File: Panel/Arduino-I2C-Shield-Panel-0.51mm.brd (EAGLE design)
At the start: 127.8 x 141 mm, 136 parts, among them Q1 200mA/50V, Q2 200mA/50V, Q3 200mA/50V, Q4 200mA/50V, Q5 200mA/50V, Q6 200mA/50V, Q7 200mA/50V, Q8 200mA/50V, U1 ARDUINO UNO, U2 ARDUINO UNO, U3 ARDUINO UNO, U4 ARDUINO UNO

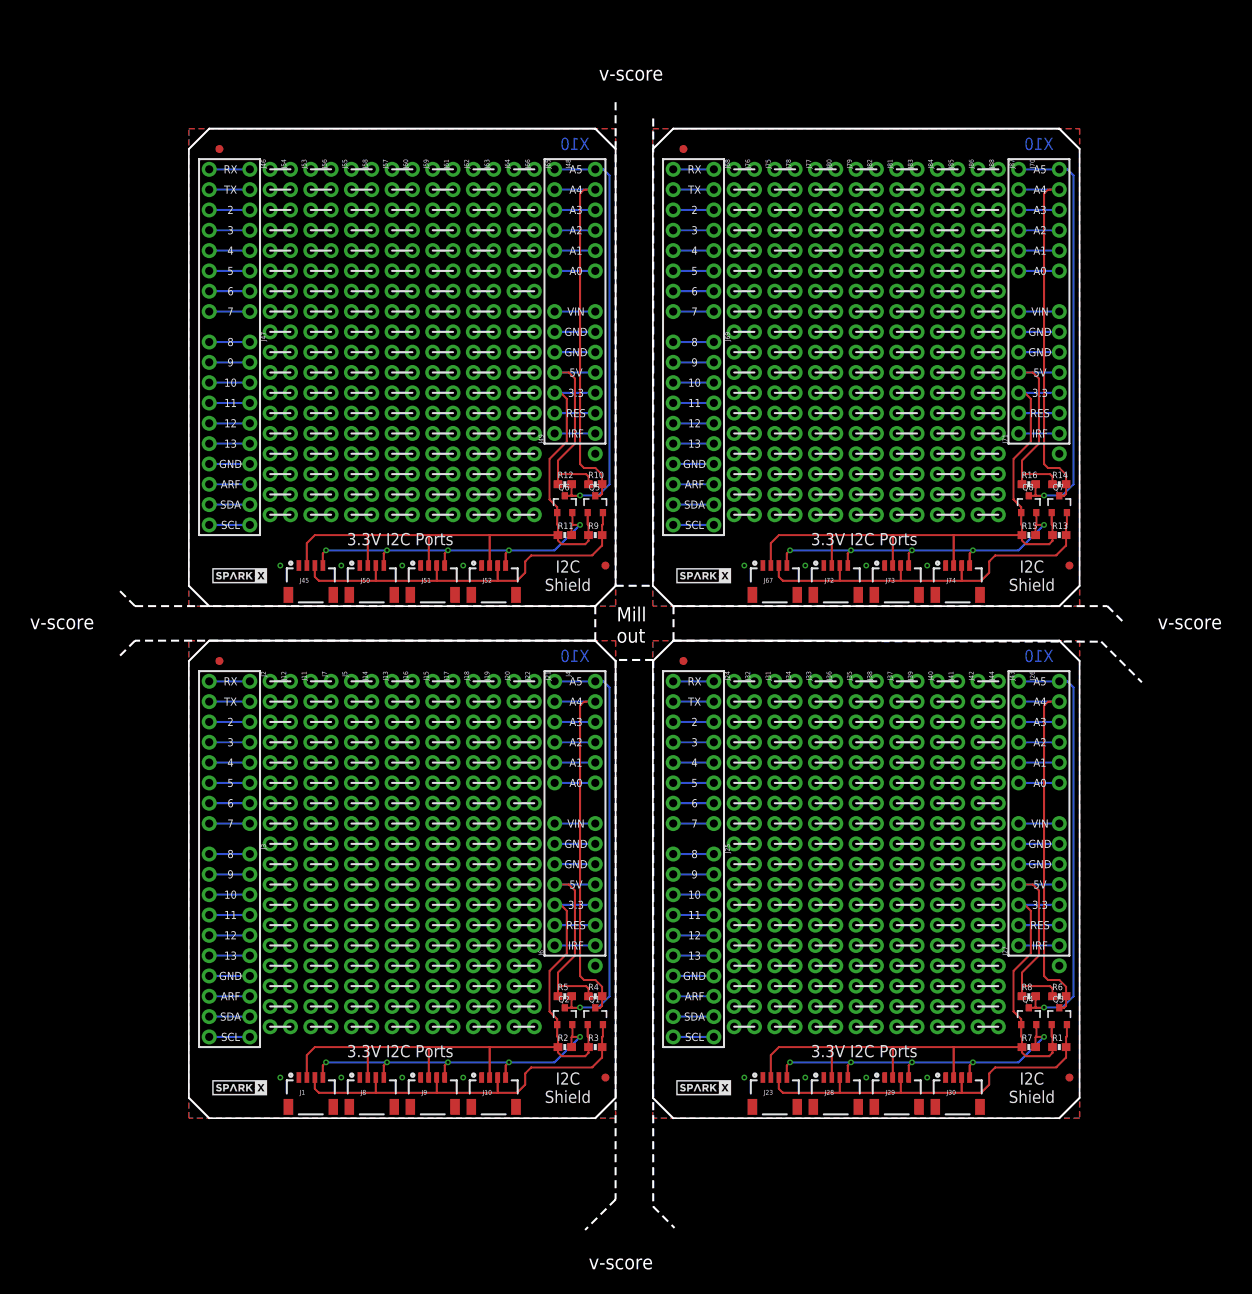
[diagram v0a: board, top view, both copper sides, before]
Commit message: Adding Mux Shield
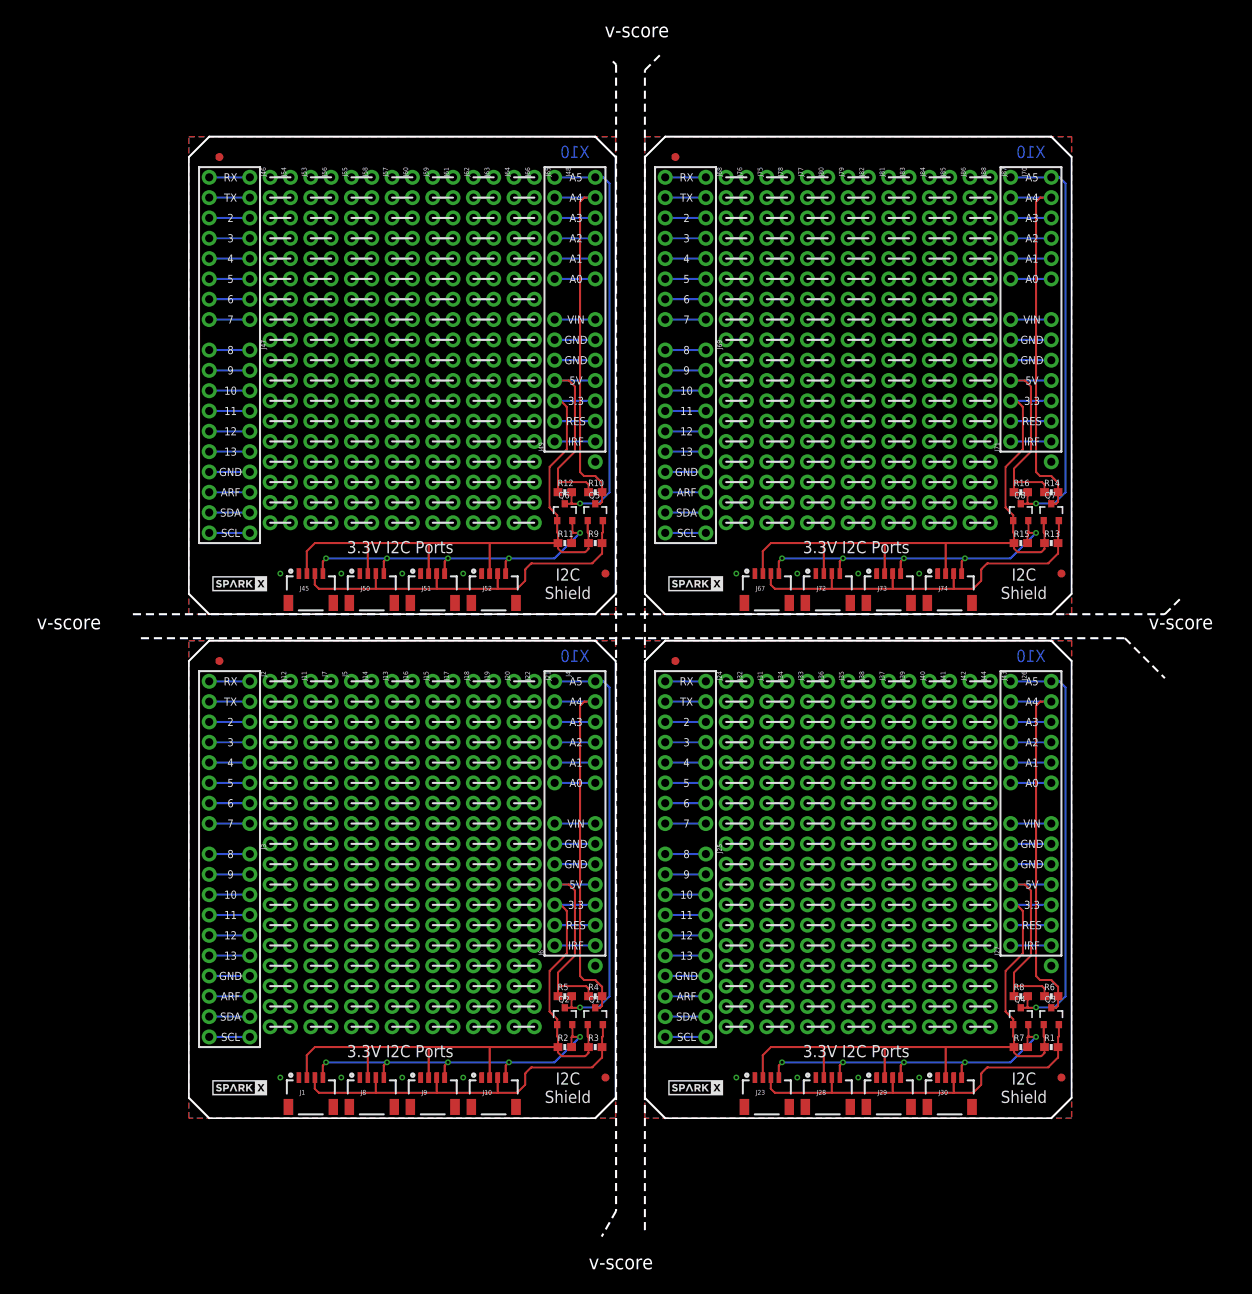
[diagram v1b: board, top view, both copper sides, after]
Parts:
- moved FD7 1.41 mm to (109.1, 68.1)
- moved FD8 1.41 mm to (60.8, 120.2)
- moved J67 1.41 mm to (72.2, 68.1)
- moved J68 1.41 mm to (64.6, 117.6)
- moved J69 1.41 mm to (64.6, 96.0)
- moved J70 1.41 mm to (102.7, 117.6)
- moved J71 1.41 mm to (102.7, 84.6)
- moved J72 1.41 mm to (79.9, 68.1)
- moved J73 1.41 mm to (87.5, 68.1)
- moved J74 1.41 mm to (95.1, 68.1)
- moved J75 1.41 mm to (69.7, 117.6)
- moved J76 1.41 mm to (67.2, 117.6)
- moved J77 1.41 mm to (74.8, 117.6)
- moved J78 1.41 mm to (72.2, 117.6)
- moved J79 1.41 mm to (79.9, 117.6)
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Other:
- board size 127.8 x 141 mm -> 131 x 147.8 mm
- board text removed: "Mill out"
